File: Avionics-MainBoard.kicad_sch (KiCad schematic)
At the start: 4 parts

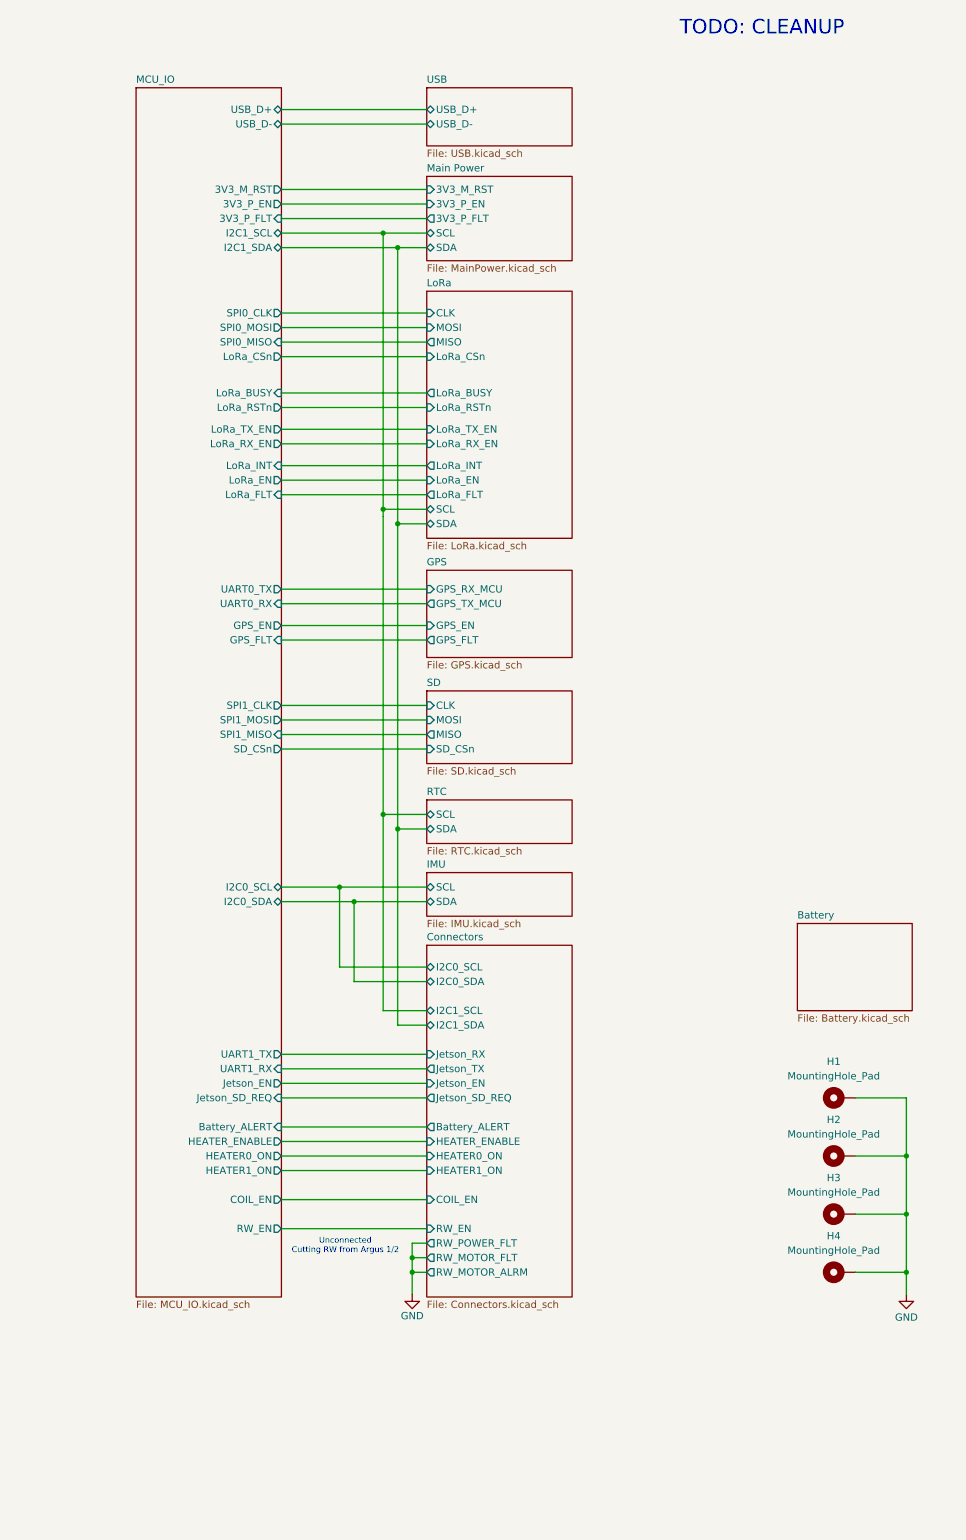
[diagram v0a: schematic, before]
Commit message: v5.0 Updates
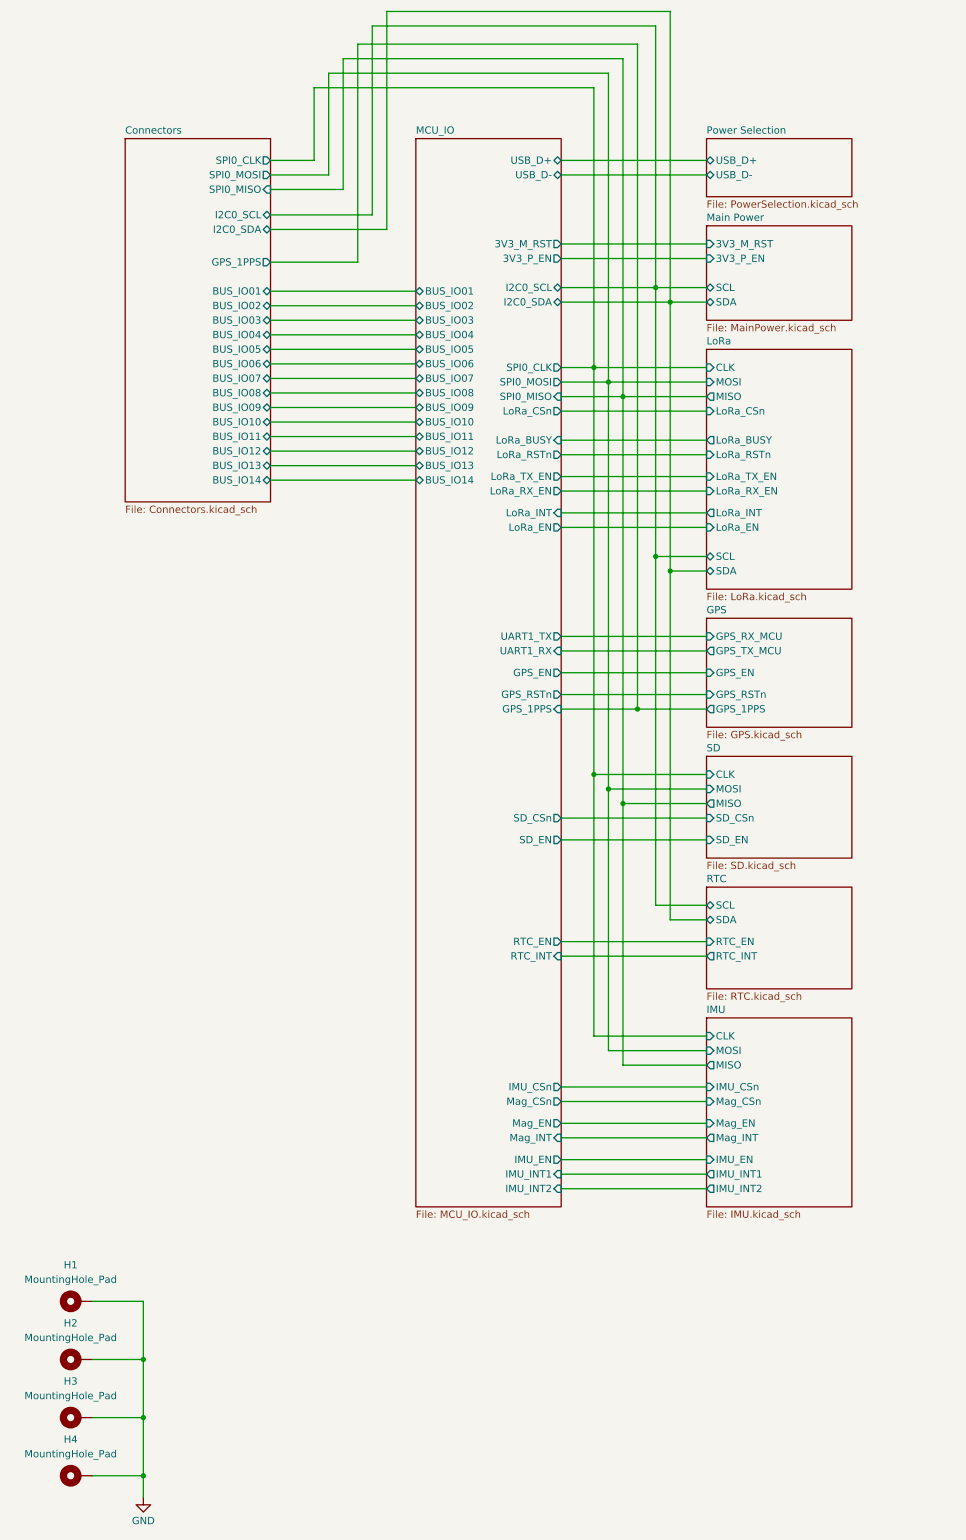
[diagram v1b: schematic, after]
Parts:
- H1, H2, H3, H4: footprint MountingHole:MountingHole_3.2mm_M3_DIN965_Pad_TopBottom -> MountingHole:MountingHole_3.2mm_M3_Pad_Via
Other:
- sheet USB renamed Power Selection
- removed sheet Battery
- sheet Connectors ports: added BUS_IO01, BUS_IO02, BUS_IO03, BUS_IO04, BUS_IO05, BUS_IO06, BUS_IO07, BUS_IO08, BUS_IO09, BUS_IO10, BUS_IO11, BUS_IO12, BUS_IO13, BUS_IO14, GPS_1PPS, SPI0_CLK, SPI0_MISO, SPI0_MOSI; removed Battery_ALERT, COIL_EN, HEATER0_ON, HEATER1_ON, HEATER_ENABLE, I2C1_SCL, I2C1_SDA, Jetson_EN, Jetson_RX, Jetson_SD_REQ, Jetson_TX, RW_EN, RW_MOTOR_ALRM, RW_MOTOR_FLT, RW_POWER_FLT
- sheet GPS ports: added GPS_1PPS, GPS_RSTn; removed GPS_FLT
- sheet IMU ports: added CLK, IMU_CSn, IMU_EN, IMU_INT1, IMU_INT2, MISO, MOSI, Mag_CSn, Mag_EN, Mag_INT; removed SCL, SDA
- sheet LoRa ports: added none; removed LoRa_FLT
- sheet MCU_IO ports: added BUS_IO01, BUS_IO02, BUS_IO03, BUS_IO04, BUS_IO05, BUS_IO06, BUS_IO07, BUS_IO08, BUS_IO09, BUS_IO10, BUS_IO11, BUS_IO12, BUS_IO13, BUS_IO14, GPS_1PPS, GPS_RSTn, IMU_CSn, IMU_EN, IMU_INT1, IMU_INT2, Mag_CSn, Mag_EN, Mag_INT, RTC_EN, RTC_INT, SD_EN; removed 3V3_P_FLT, Battery_ALERT, COIL_EN, GPS_FLT, HEATER0_ON, HEATER1_ON, HEATER_ENABLE, I2C1_SCL, I2C1_SDA, Jetson_EN, Jetson_SD_REQ, LoRa_FLT, RW_EN, SPI1_CLK, SPI1_MISO, SPI1_MOSI, UART0_RX, UART0_TX
- sheet Main Power ports: added none; removed 3V3_P_FLT
- sheet Power Selection: file USB.kicad_sch -> PowerSelection.kicad_sch
- sheet RTC ports: added RTC_EN, RTC_INT; removed none
- sheet SD ports: added SD_EN; removed none
- note removed: "TODO: CLEANUP"
- note removed: "Unconnected Cutting RW from Argus 1/2"
- moved on the sheet: H1, H2, H3, H4
